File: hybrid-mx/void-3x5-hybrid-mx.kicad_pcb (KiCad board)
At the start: 2 copper layers, 140.5 x 112.5 mm, 82 parts, among them J1 USB_C_Receptacle_PowerOnly_6P, J2 Conn_01x02, J3 Conn_01x02, J4 Conn_01x03

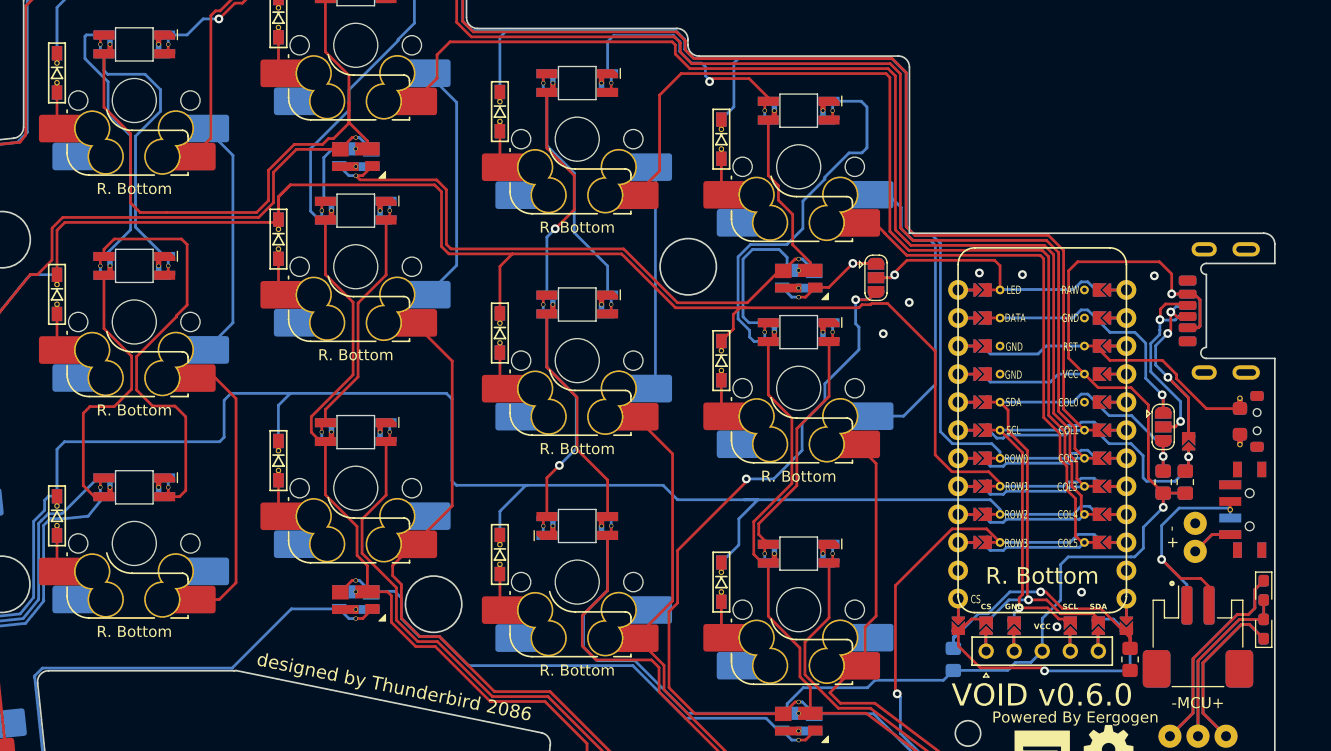
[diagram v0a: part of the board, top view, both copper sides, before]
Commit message: updated choc
* fixed corner
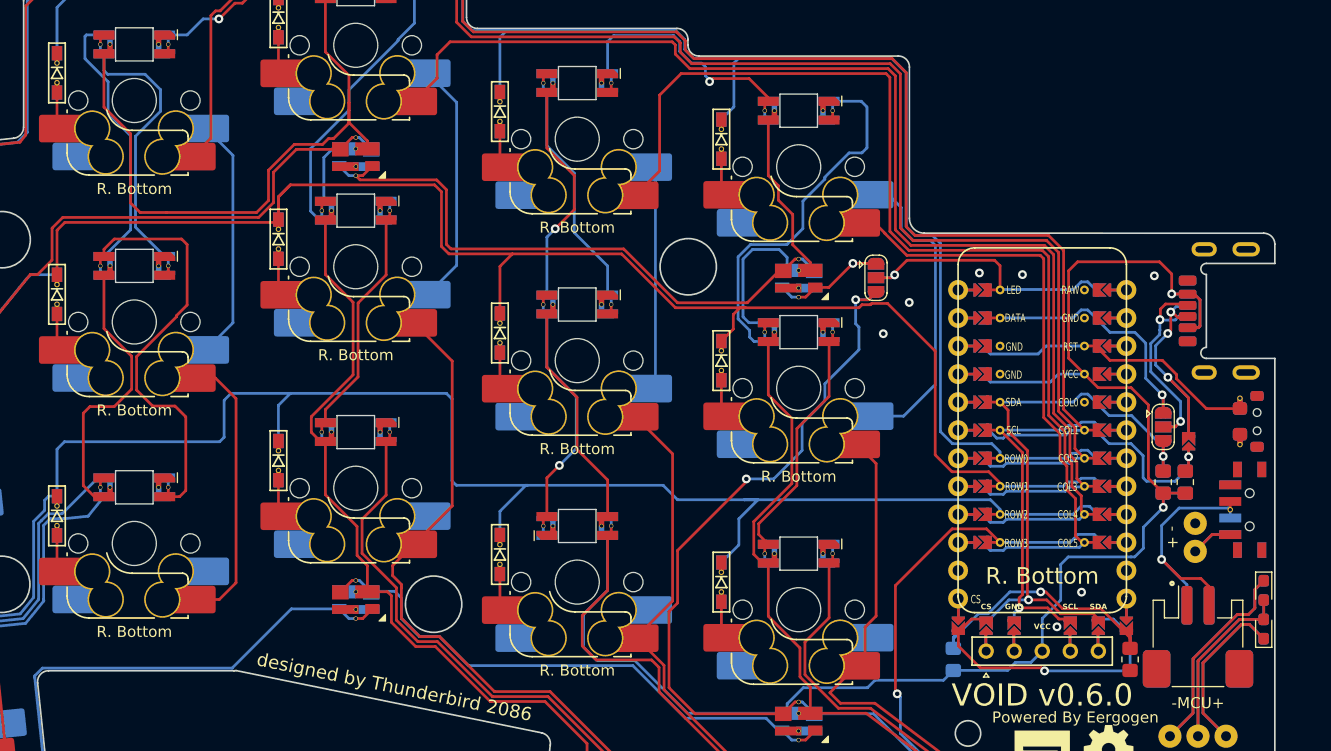
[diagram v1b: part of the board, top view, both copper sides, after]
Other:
- outline, holes or cut-outs redrawn
- board text added: "This corner was manually created."
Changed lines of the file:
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@@
 		(fp_arc
 			(start 4.085176 -6.75022)
-			(mid 5.499389 -6.164434)
+			(mid 5.499392 -6.164435)
 			(end 6.085176 -4.75022)
 			(stroke
@@
 		(fp_arc
 			(start 4.085176 -6.75022)
-			(mid 5.499389 -6.164434)
+			(mid 5.499392 -6.164435)
 			(end 6.085176 -4.75022)
 			(stroke
@@
 		)
 		(pad "1" thru_hole circle
-			(at -2.200002 0 353)
+			(at -2.200003 0 353)
 			(size 0.4 0.4)
 			(drill 0.3)
@@
 		)
 		(pad "3" thru_hole circle
-			(at 2.200002 0 353)
+			(at 2.200003 0 353)
 			(size 0.4 0.4)
 			(drill 0.3)
@@
 		(fp_arc
 			(start 4.085176 -6.75022)
-			(mid 5.499389 -6.164434)
+			(mid 5.499392 -6.164435)
 			(end 6.085176 -4.75022)
 			(stroke
@@
 		(fp_arc
 			(start 4.085176 -6.75022)
-			(mid 5.499389 -6.164434)
+			(mid 5.499392 -6.164435)
 			(end 6.085176 -4.75022)
 			(stroke
@@
 		(fp_arc
 			(start 4.085176 -6.75022)
-			(mid 5.499389 -6.164434)
+			(mid 5.499392 -6.164435)
 			(end 6.085176 -4.75022)
 			(stroke
@@
 		(fp_arc
 			(start 4.085176 -6.75022)
-			(mid 5.499389 -6.164434)
+			(mid 5.499392 -6.164435)
 			(end 6.085176 -4.75022)
 			(stroke
@@
 		(fp_arc
 			(start 4.085176 -6.75022)
-			(mid 5.499389 -6.164434)
+			(mid 5.499392 -6.164435)
 			(end 6.085176 -4.75022)
 			(stroke
@@
 		(fp_arc
 			(start 4.085176 -6.75022)
-			(mid 5.499389 -6.164434)
+			(mid 5.499392 -6.164435)
 			(end 6.085176 -4.75022)
 			(stroke
@@
 		(tags "resistor handsolder")
 		(property "Reference" "R2"
-			(at 0 -1.65 270)
+			(at 0 -1.65 -90)
 			(layer "F.SilkS")
 			(hide yes)
@@
 		(fp_arc
 			(start 4.085176 -6.75022)
-			(mid 5.499389 -6.164434)
+			(mid 5.499392 -6.164435)
 			(end 6.085176 -4.75022)
 			(stroke
@@
 		(fp_arc
 			(start 4.085176 -6.75022)
-			(mid 5.499389 -6.164434)
+			(mid 5.499392 -6.164435)
 			(end 6.085176 -4.75022)
 			(stroke
@@
 		(fp_arc
 			(start 4.085176 -6.75022)
-			(mid 5.499389 -6.164434)
+			(mid 5.499392 -6.164435)
 			(end 6.085176 -4.75022)
 			(stroke
@@
 		(fp_arc
 			(start 4.085176 -6.75022)
-			(mid 5.499389 -6.164434)
+			(mid 5.499392 -6.164435)
 			(end 6.085176 -4.75022)
 			(stroke
@@
 		(fp_arc
 			(start -2.444146 -0.85)
-			(mid -1.620516 -2.173416)
+			(mid -1.620517 -2.173415)
 			(end -0.149824 -2.69)
 			(stroke
@@
 		(fp_arc
 			(start 4.085176 -6.75022)
-			(mid 5.499389 -6.164435)
+			(mid 5.499392 -6.164435)
 			(end 6.085176 -4.75022)
 			(stroke
@@
 		(fp_line
 			(start 7.465 -6.31)
-			(end 4.915002 -6.31)
+			(end 4.915003 -6.31)
 			(stroke
 				(width 0.05)
@@
 		(fp_line
 			(start 4.915 -6.74)
-			(end 4.915002 -6.31)
+			(end 4.915003 -6.31)
 			(stroke
 				(width 0.05)
@@
 		(fp_arc
 			(start 4.085176 -6.75022)
-			(mid 5.499389 -6.164435)
+			(mid 5.499392 -6.164435)
 			(end 6.085176 -4.75022)
 			(stroke
@@
 		(fp_arc
 			(start 4.085176 -6.75022)
-			(mid 5.499389 -6.164434)
+			(mid 5.499392 -6.164435)
 			(end 6.085176 -4.75022)
 			(stroke
@@
 		(fp_arc
 			(start 4.085176 -6.75022)
-			(mid 5.499389 -6.164434)
+			(mid 5.499392 -6.164435)
 			(end 6.085176 -4.75022)
 			(stroke
@@
 		(fp_arc
 			(start 4.085176 -6.75022)
-			(mid 5.499389 -6.164434)
+			(mid 5.499392 -6.164435)
 			(end 6.085176 -4.75022)
 			(stroke
@@
 		(fp_arc
 			(start 4.085176 -6.75022)
-			(mid 5.499389 -6.164434)
+			(mid 5.499392 -6.164435)
 			(end 6.085176 -4.75022)
 			(stroke
@@
 		(fp_arc
 			(start -3.4 1.475)
-			(mid -2.826424 1.655849)
+			(mid -2.826425 1.655849)
 			(end -2.460307 2.13298)
 			(stroke
@@
 		(fp_arc
 			(start -0.299999 3.624999)
-			(mid -1.577272 3.167235)
+			(mid -1.577271 3.167235)
 			(end -2.455444 2.13293)
 			(stroke
@@
 		(fp_arc
 			(start 2.455444 2.13293)
-			(mid 1.577273 3.167237)
+			(mid 1.577274 3.167237)
 			(end 0.299999 3.624997)
 			(stroke
@@
 		(at 154.701652 93.836424 180)
 		(property "Reference" "L10"
-			(at 0 2.1 360)
+			(at 0 2.1 0)
 			(layer "Eco1.User")
 			(effects
@@
 		)
 		(property "Value" "SK6812MINI-E"
-			(at 0 -0.5 360)
+			(at 0 -0.5 0)
 			(layer "B.SilkS")
 			(hide yes)
@@
 		)
 		(property "Footprint" "TB2086_LED:LED_SK6812MINI-E_rev"
-			(at 0 0 360)
+			(at 0 0 0)
 			(layer "F.Fab")
 			(hide yes)
@@
 		)
 		(property "Datasheet" "https://cdn-shop.adafruit.com/product-files/2686/SK6812MINI_REV.01-1-2.pdf"
-			(at 0 0 360)
+			(at 0 0 0)
 			(layer "F.Fab")
 			(hide yes)
@@
 		)
 		(property "Description" ""
-			(at 0 0 360)
+			(at 0 0 0)
 			(layer "F.Fab")
 			(hide yes)
@@
 		(fp_arc
 			(start 4.085176 -6.75022)
-			(mid 5.499389 -6.164434)
+			(mid 5.499392 -6.164435)
 			(end 6.085176 -4.75022)
 			(stroke
@@
 		(fp_arc
 			(start 4.085176 -6.75022)
-			(mid 5.499389 -6.164434)
+			(mid 5.499392 -6.164435)
 			(end 6.085176 -4.75022)
 			(stroke
@@
 		(fp_arc
 			(start -2.444146 -0.85)
-			(mid -1.620516 -2.173416)
+			(mid -1.620517 -2.173415)
 			(end -0.149824 -2.69)
 			(stroke
@@
 		(fp_arc
 			(start 4.085176 -6.75022)
-			(mid 5.499389 -6.164435)
+			(mid 5.499392 -6.164435)
 			(end 6.085176 -4.75022)
 			(stroke
@@
 		(fp_line
 			(start 7.465 -6.31)
-			(end 4.915002 -6.31)
+			(end 4.915003 -6.31)
 			(stroke
 				(width 0.05)
@@
 		(fp_line
 			(start 4.915 -6.74)
-			(end 4.915002 -6.31)
+			(end 4.915003 -6.31)
 			(stroke
 				(width 0.05)
@@
 		(fp_arc
 			(start 4.085176 -6.75022)
-			(mid 5.499389 -6.164435)
+			(mid 5.499392 -6.164435)
 			(end 6.085176 -4.75022)
 			(stroke
@@
 		(fp_arc
 			(start 4.085176 -6.75022)
-			(mid 5.499389 -6.164434)
+			(mid 5.499392 -6.164435)
 			(end 6.085176 -4.75022)
 			(stroke
@@
 		(fp_arc
 			(start 4.085176 -6.75022)
-			(mid 5.499389 -6.164434)
+			(mid 5.499392 -6.164435)
 			(end 6.085176 -4.75022)
 			(stroke
@@
 		(fp_arc
 			(start 4.085176 -6.75022)
-			(mid 5.499389 -6.164434)
+			(mid 5.499392 -6.164435)
 			(end 6.085176 -4.75022)
 			(stroke
@@
 		(fp_arc
 			(start 4.085176 -6.75022)
-			(mid 5.499389 -6.164434)
+			(mid 5.499392 -6.164435)
 			(end 6.085176 -4.75022)
 			(stroke
@@
 		(fp_arc
 			(start 4.085176 -6.75022)
-			(mid 5.499389 -6.164434)
+			(mid 5.499392 -6.164435)
 			(end 6.085176 -4.75022)
 			(stroke
@@
 		(fp_arc
 			(start 4.085176 -6.75022)
-			(mid 5.499389 -6.164434)
+			(mid 5.499392 -6.164435)
 			(end 6.085176 -4.75022)
 			(stroke
@@
 		(fp_arc
 			(start -6.95 -6.45)
-			(mid -6.803553 -6.803552)
+			(mid -6.803552 -6.803552)
 			(end -6.45 -6.95)
 			(stroke
@@
 		(fp_arc
 			(start -6.45 6.95)
-			(mid -6.803552 6.803553)
+			(mid -6.803552 6.803552)
 			(end -6.95 6.45)
 			(stroke
@@
 		(fp_arc
 			(start -3.45 6.125001)
-			(mid -2.742894 6.417893)
+			(mid -2.742893 6.417893)
 			(end -2.45 7.125)
 			(stroke
@@
 		(fp_arc
 			(start -2.444146 -0.85)
-			(mid -1.620516 -2.173416)
+			(mid -1.620517 -2.173415)
 			(end -0.149824 -2.69)
 			(stroke
@@
 		(fp_arc
 			(start 4.085176 -6.75022)
-			(mid 5.499389 -6.164435)
+			(mid 5.499392 -6.164435)
 			(end 6.085176 -4.75022)
 			(stroke
@@
 		(fp_line
 			(start 7.465 -6.31)
-			(end 4.915002 -6.31)
+			(end 4.915003 -6.31)
 			(stroke
 				(width 0.05)
@@
 		(fp_line
 			(start 4.915 -6.74)
-			(end 4.915002 -6.31)
+			(end 4.915003 -6.31)
 			(stroke
 				(width 0.05)
@@
 		(fp_arc
 			(start 4.085176 -6.75022)
-			(mid 5.499389 -6.164435)
+			(mid 5.499392 -6.164435)
 			(end 6.085176 -4.75022)
 			(stroke
@@
 	(gr_line
 		(start 216.859152 67.331424)
-		(end 184.776652 67.331424)
+		(end 186.122009 67.324289)
 		(stroke
 			(width 0.15)
@@
 		(layer "Edge.Cuts")
 	)
+	(gr_arc
+		(start 186.122009 67.324289)
+		(mid 185.17 66.93)
+		(end 184.775711 65.977991)
+		(stroke
+			(width 0.15)
+			(type default)
+		)
+		(layer "Edge.Cuts")
+	)
 	(gr_circle
 		(center 102.601652 99.116424)
@@
 	)
 	(gr_line
-		(start 184.776652 67.331424)
+		(start 184.775711 65.977991)
 		(end 184.776652 52.291424)
 		(stroke
@@
 		)
 	)
+	(gr_text "This corner was manually created. "
+		(at 185.45 66.63 0)
+		(layer "Cmts.User")
+		(effects
+			(font
+				(size 1 1)
+				(thickness 0.15)
+			)
+			(justify left bottom)
+		)
+	)

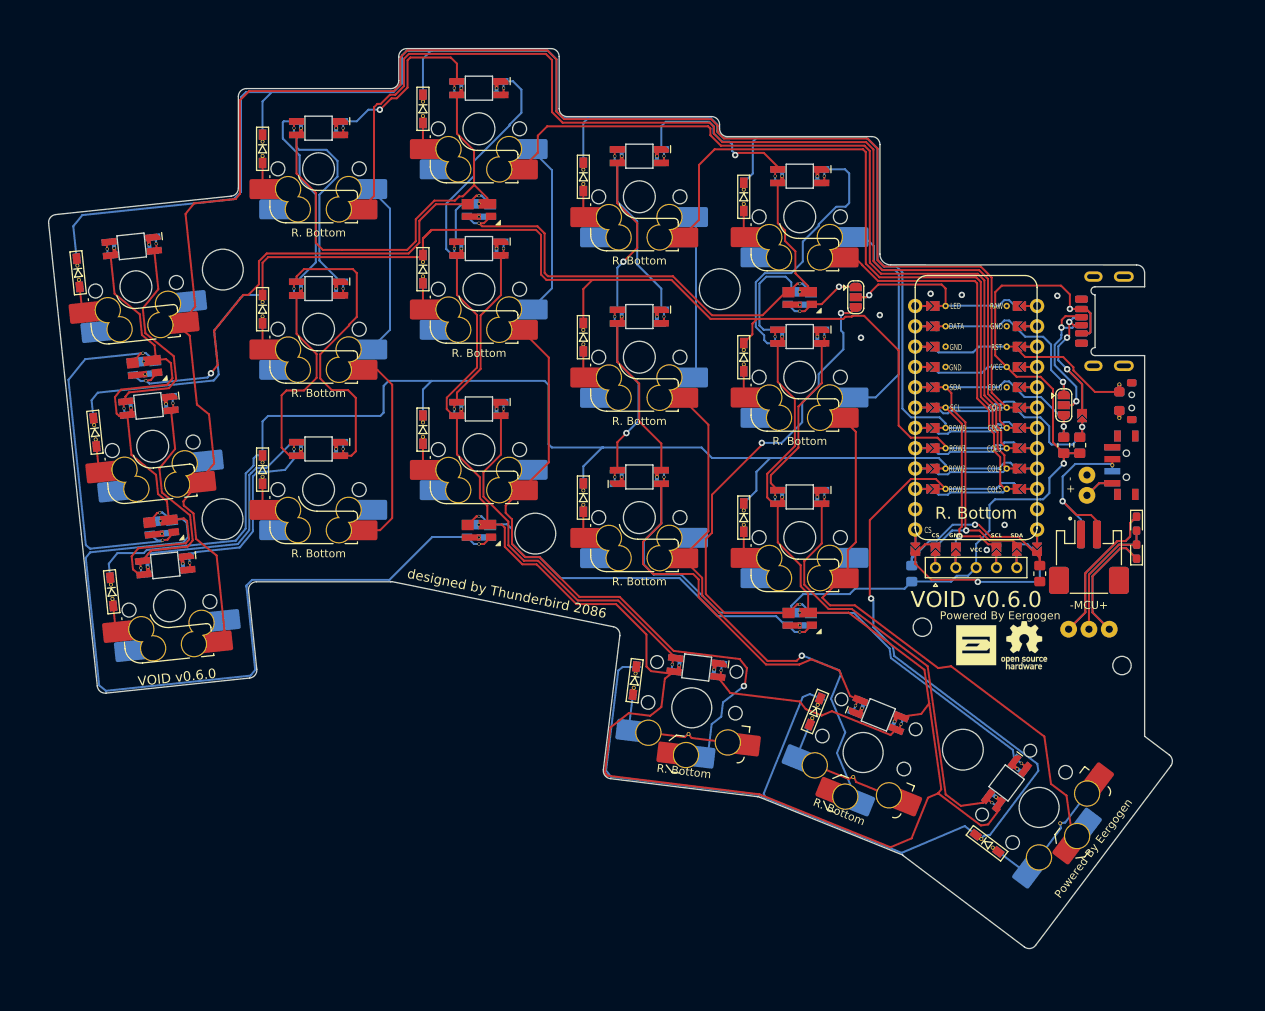
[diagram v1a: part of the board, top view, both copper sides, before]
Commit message: updated PCBs
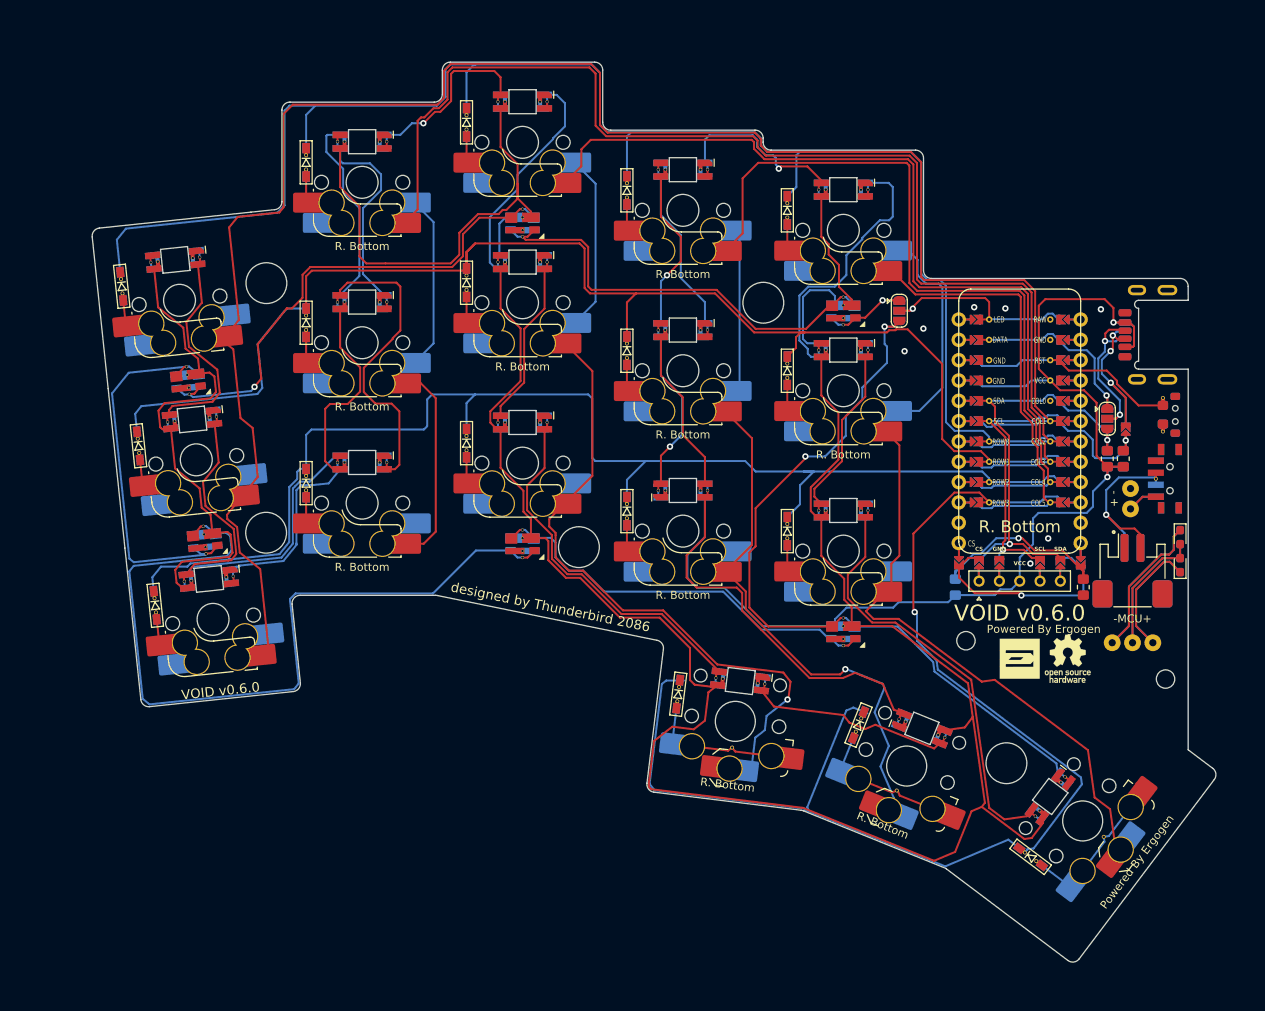
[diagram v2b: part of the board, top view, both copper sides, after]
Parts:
- moved D8 5.70 mm to (133.1, 69.6)
- moved D9 5.70 mm to (133.1, 49.5)
- moved D2 5.70 mm to (92.1, 89.9)
- moved D7 5.70 mm to (133.1, 89.6)
- moved D11 5.70 mm to (153.1, 78.1)
- moved D14 5.70 mm to (173.2, 80.6)
- moved D16 5.70 mm to (159.6, 121.0)
- moved D17 5.70 mm to (182.1, 124.8)
- moved D18 5.70 mm to (203.6, 141.3)
- moved D3 5.70 mm to (90.0, 70.0)
- moved D5 5.70 mm to (113.0, 74.6)
- moved J1 5.70 mm to (219.9, 76.1)
- moved J2 5.70 mm to (216.3, 105.6)
- moved J3 5.70 mm to (216.1, 96.6)
- moved J4 5.70 mm to (216.3, 114.6)
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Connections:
- RSW1 pad MP: GND -> (no net)
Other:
- outline, holes or cut-outs redrawn
- board text added: "Powered By Ergogen"
- board text added: "offset: 90, 70 from origin"
- board text removed: "Powered By Eergogen"
- board text removed: "This corner was manually created."
